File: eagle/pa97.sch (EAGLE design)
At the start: 34 parts

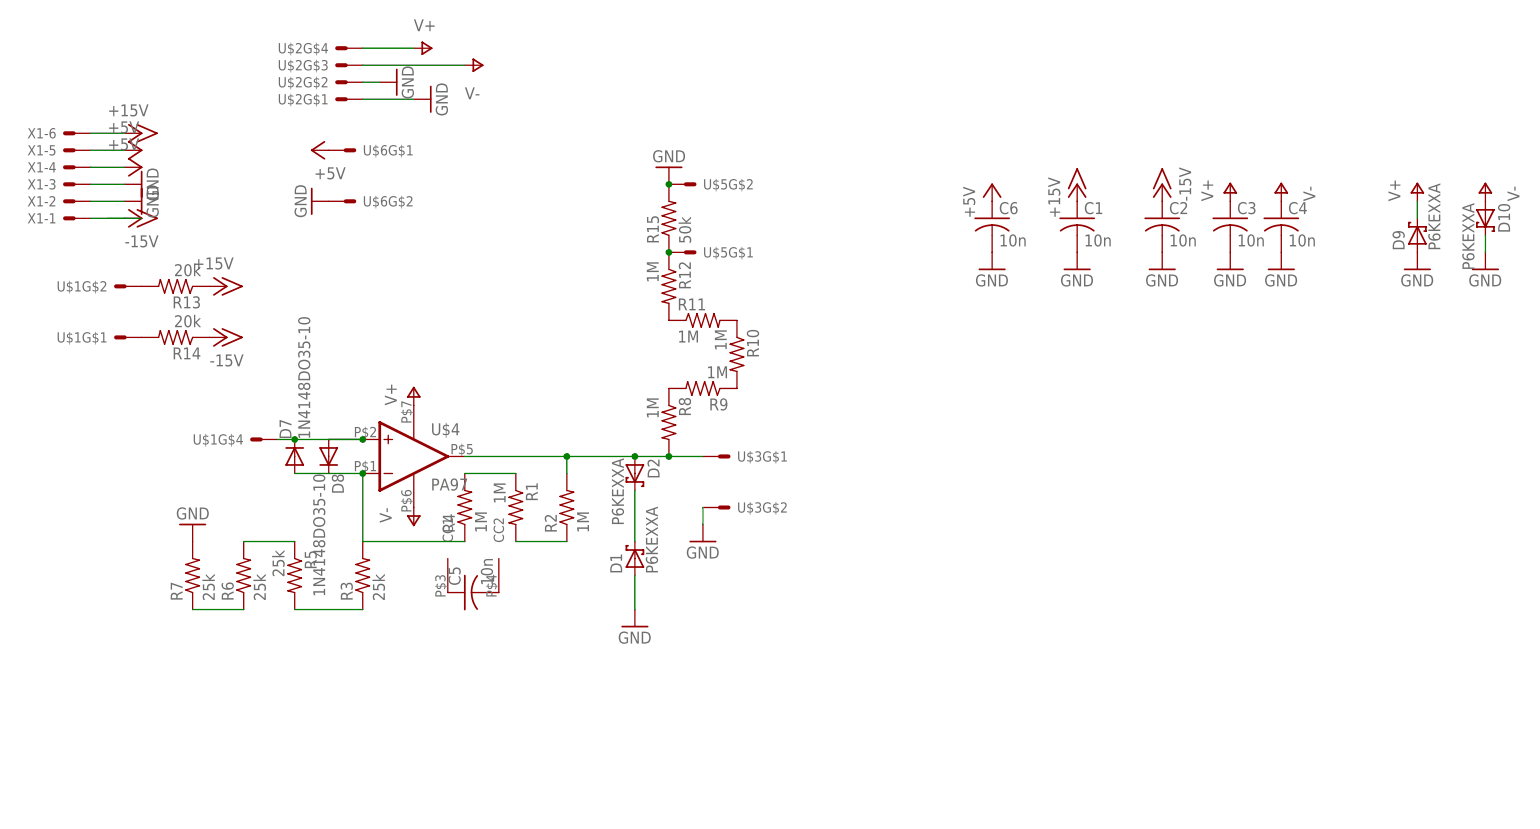
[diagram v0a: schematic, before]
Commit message: Test layouts pa97
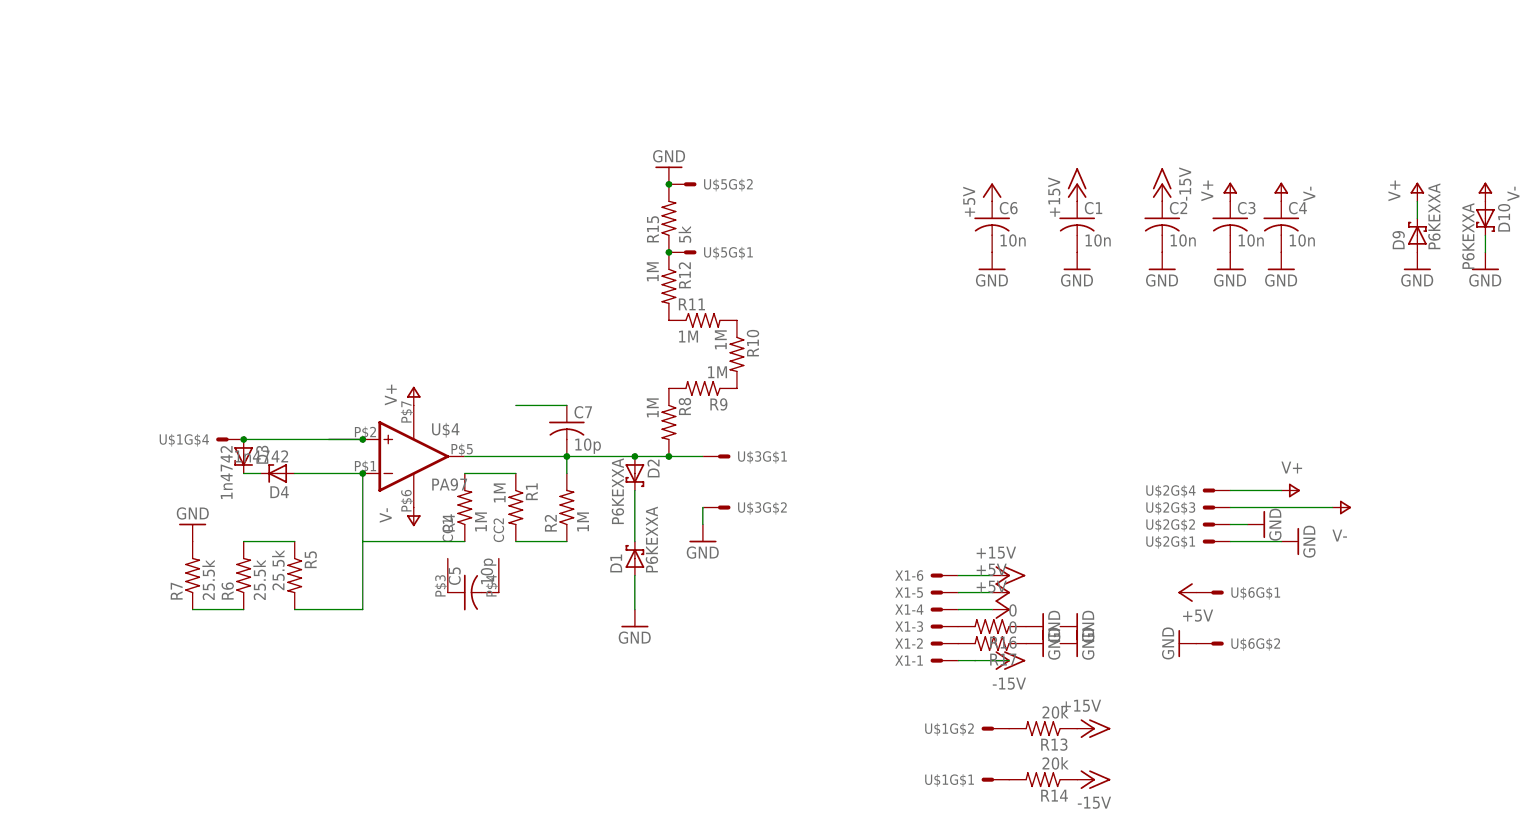
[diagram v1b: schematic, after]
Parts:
- removed D7, D8: 1N4148DO35-10, diode:1N4148DO35-10
- removed R3: 25k, rcl:R-US_0207/10
- added C7: 10p, rcl:C-US075-032X103
- added D3, D4: 1n4742, diode:ZENER-DIODEDO41Z10
- added R16, R17: 0, rcl:R-US_0207/10
- C5: value 10n -> 10p
- R15: value 50k -> 5k
- R5, R6, R7: value 25k -> 25.5k
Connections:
- new net N$18: R16.2, X1-3.S
- new net N$19: R17.2, X1-2.S
- new net N$20: D3.C, D4.C
- net GND: now also R16.1, R17.1; no longer X1-2.S, X1-3.S
- net N$10: now also C7.1; no longer D7.A, D8.C, R3.2, R4.1, U$4.-IN
- net N$11: now also C7.2
- net N$13: now also D3.A; no longer D7.C, D8.A
- net N$3: now also D4.A, R4.1, U$4.-IN; no longer R3.1
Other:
- moved on the sheet: R13, R14, U$1G$1, U$1G$2, U$1G$4, U$2G$1, U$2G$2, U$2G$3, U$2G$4, U$6G$1, U$6G$2, X1-1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
